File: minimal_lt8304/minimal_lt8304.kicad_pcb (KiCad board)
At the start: 4 copper layers, 63.9 x 22.9 mm, 41 parts, among them J1 FW-02-03-G-D-085-155, J2 FW-02-03-G-D-085-155, J3 FW-02-03-G-D-085-155, J4 FW-02-03-G-D-085-155, T1 750315836, U1 LT8304IS8E-PBF

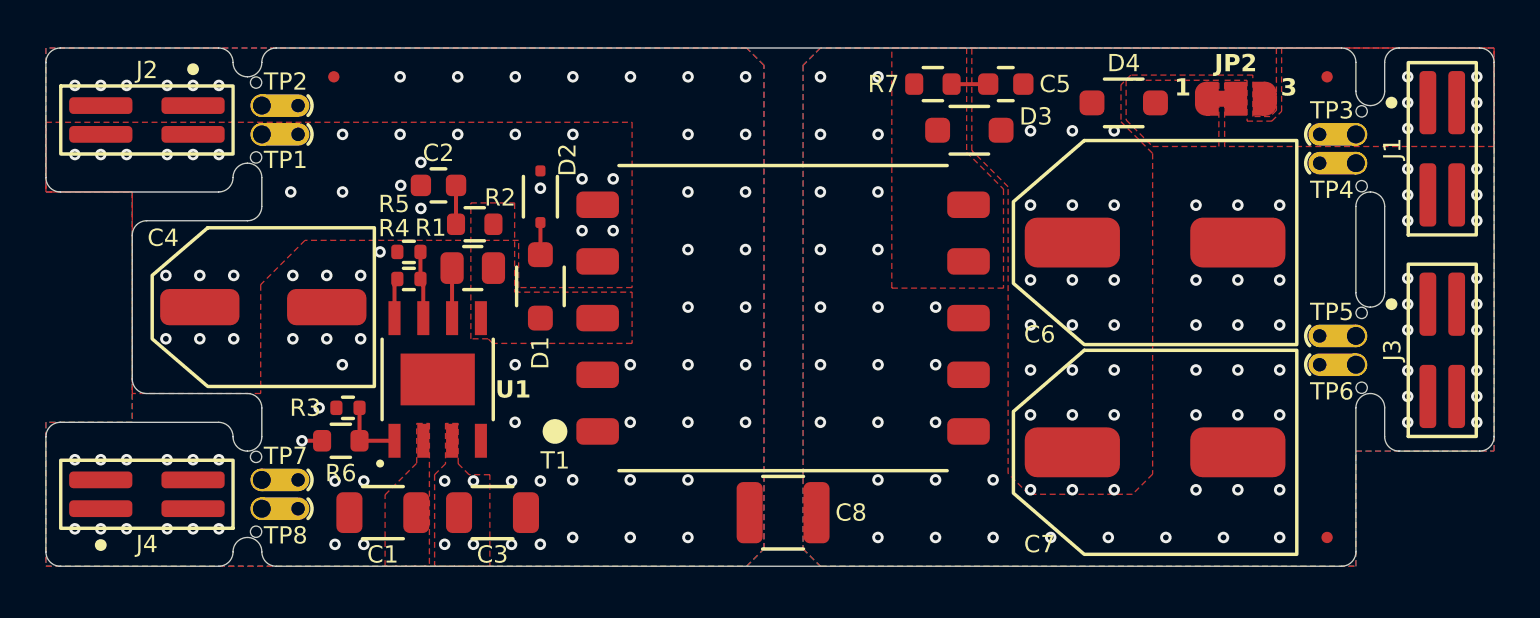
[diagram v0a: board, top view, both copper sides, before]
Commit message: update project
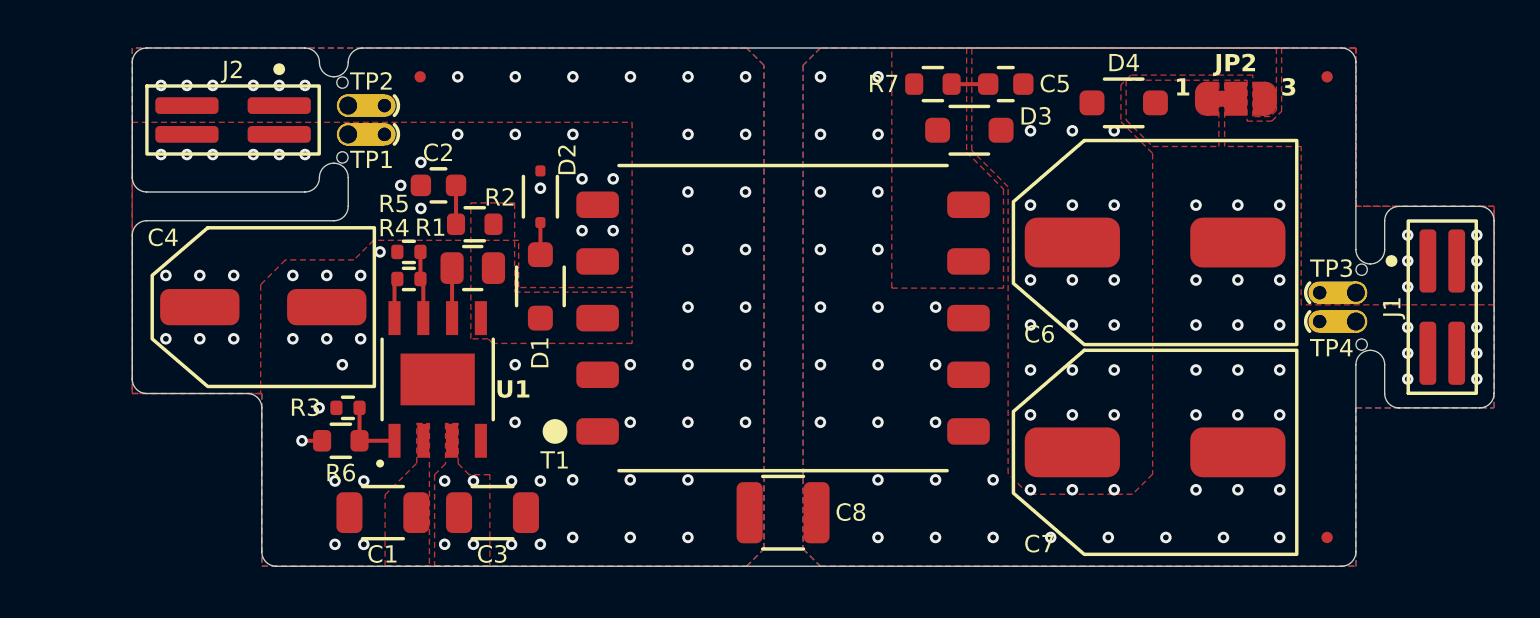
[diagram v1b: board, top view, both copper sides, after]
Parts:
- removed J3, J4: FW-02-03-G-D-085-155, connector_footprints:FW-02-03-G-D-085-155
- removed MB3, MB4: mouse-bite-midle-50mil-200mil, mouse_bite_footprints:mouse-bite-midle-50mil-200mil
- removed TP5, TP6, TP7, TP8: TestPoint, test_point_footprints:TestPoint_THTPad_Castelated
- moved J1 6.98 mm to (195.5, 112.1)
- moved MB2 6.98 mm to (192.4, 112.1)
- moved TP3 6.98 mm to (191.7, 111.4)
- moved TP4 6.98 mm to (191.7, 112.7)
- moved FID2 3.81 mm to (150.4, 101.9)
- moved MB1 3.81 mm to (146.6, 103.8)
- moved TP1 3.81 mm to (147.3, 104.4)
- moved TP2 3.81 mm to (147.3, 103.2)
- moved J2 3.80 mm to (142.2, 103.8)
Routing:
- net GNDA: vias 64 -> 52
- net GND: vias 64 -> 51
- net /VIN: vias 32 -> 28
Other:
- board size 63.9 x 22.9 mm -> 60.1 x 22.9 mm
